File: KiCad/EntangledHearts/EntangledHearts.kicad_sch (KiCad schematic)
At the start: 42 parts, among them J1 OLED Display, J2 MPU, Q1 SFH_3711, U1 ESP32-S3-WROOM-1

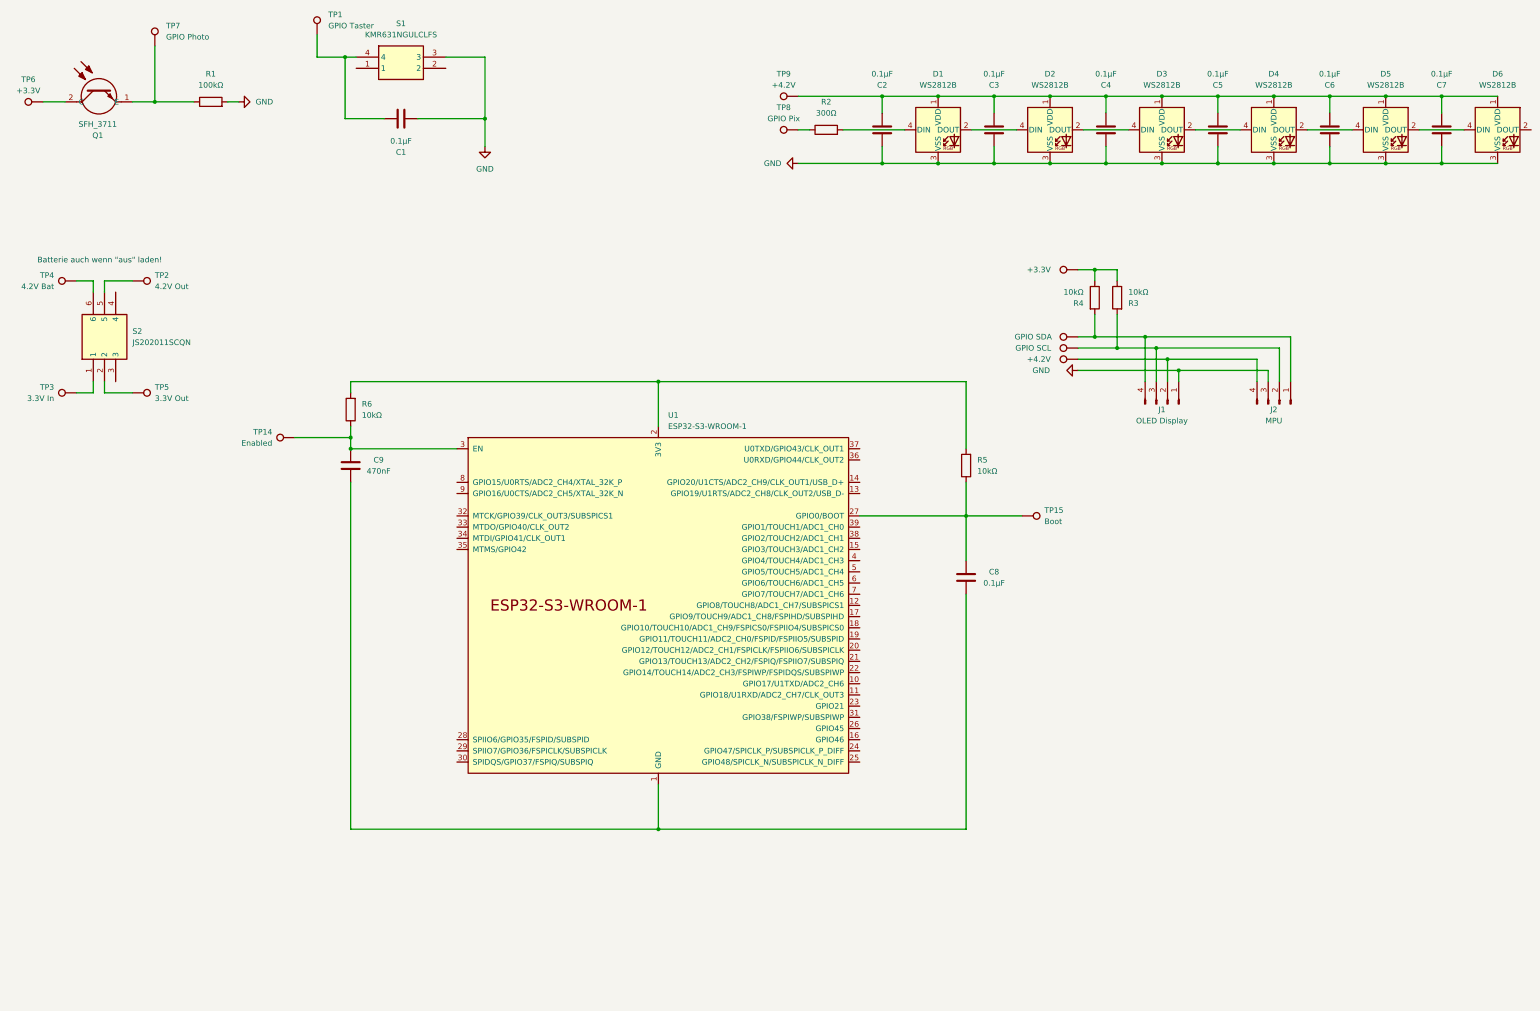
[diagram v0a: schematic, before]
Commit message: ADD: all parts added
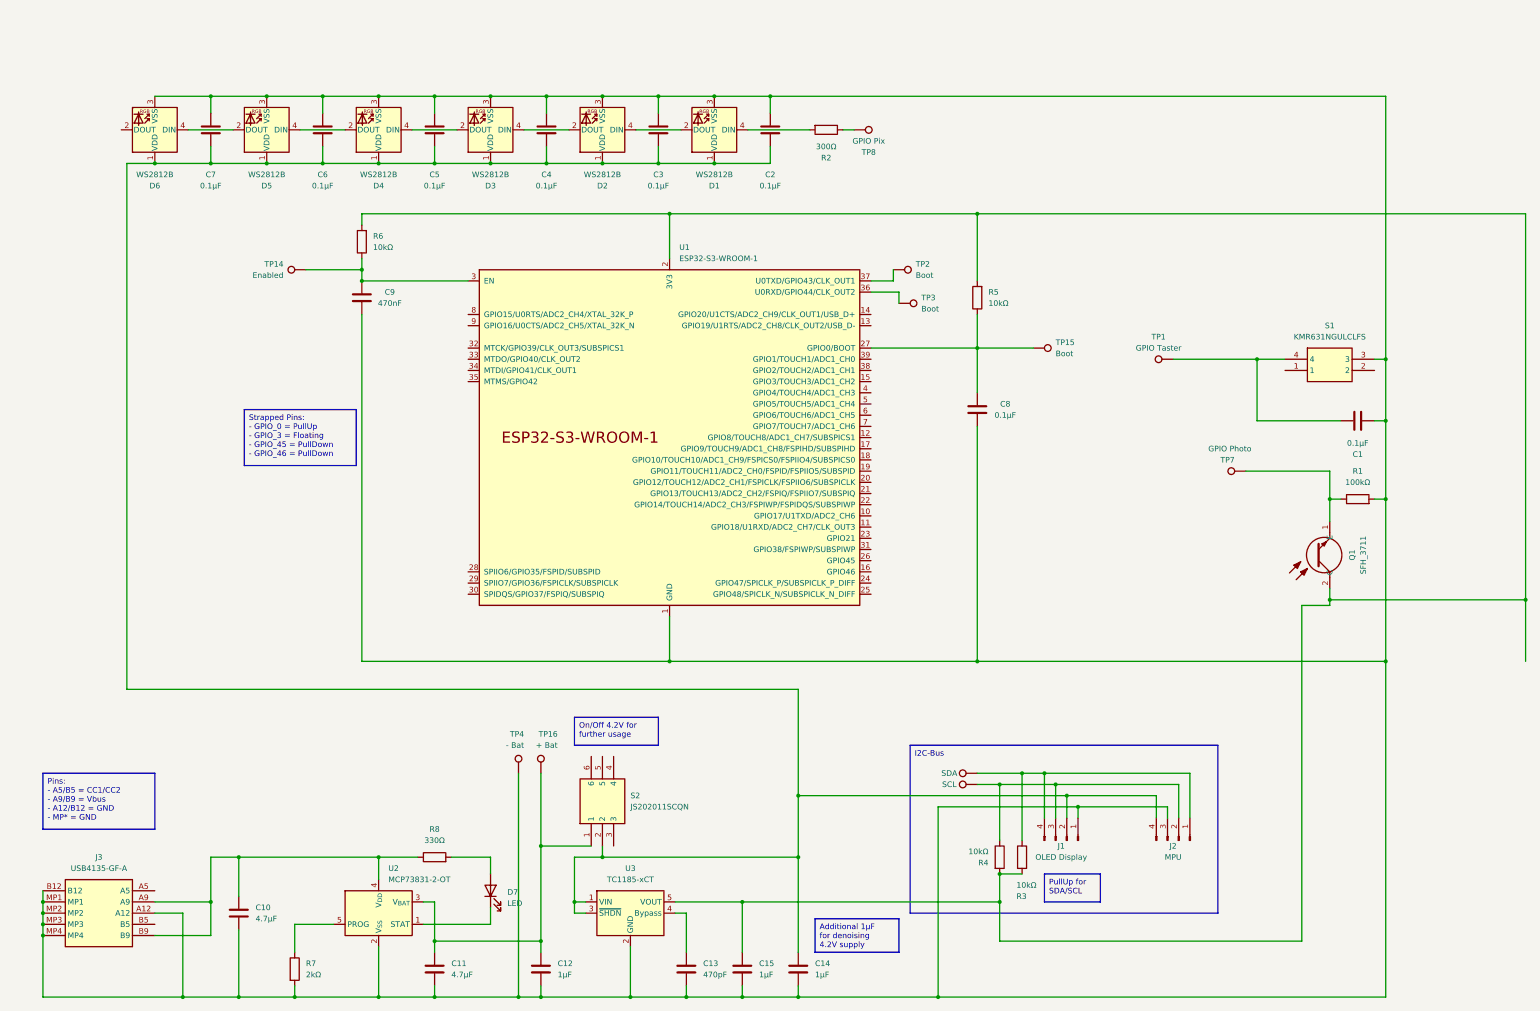
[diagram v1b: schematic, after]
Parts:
- removed TP10, TP9: +4.2V, symbol Connector:TestPoint
- removed TP13, TP6: +3.3V, symbol Connector:TestPoint
- removed TP5: 3.3V Out, symbol Connector:TestPoint
- added C10, C11: 4.7µF, symbol Device:C
- added C12, C14, C15: 1µF, symbol Device:C
- added C13: 470pF, symbol Device:C
- added D7: LED, symbol Device:LED
- added J3: USB4135-GF-A, USB4135GFA, symbol USB4135-GF-A:USB4135-GF-A
- added R7: 2kΩ, symbol Device:R
- added R8: 330Ω, symbol Device:R
- added TP16: + Bat, symbol Connector:TestPoint
- added U2: MCP73831-2-OT, Package_TO_SOT_SMD:SOT-23-5, symbol Battery_Management:MCP73831-2-OT
- added U3: TC1185-xCT, Package_TO_SOT_SMD:SOT-23-5, symbol Regulator_Linear:TC1185-xCT
- TP11: value GPIO SCL -> SCL
- TP12: value GPIO SDA -> SDA
- TP2: value 4.2V Out -> Boot
- TP3: value 3.3V In -> Boot
- TP4: value 4.2V Bat -> - Bat
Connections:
- net GND is gone; now on an unnamed net: C1.2, C2.2, C3.2, C4.2, C5.2, C6.2, C7.2, D1.3 (VSS), D2.3 (VSS), D3.3 (VSS), D4.3 (VSS), D5.3 (VSS), D6.3 (VSS), J1.1 (Pin_1), J2.3 (Pin_3), R1.2, S1.3
- net at TP2.1: now also U1.37 (U0TXD/GPIO43/CLK_OUT1); no longer S2.5
- net at J1.3 (Pin_3), J2.2 (Pin_2), TP11.1: now also R4.1; no longer R3.2
- net at J1.2 (Pin_2), J2.4 (Pin_4): now also C2.1, C3.1, C4.1, C5.1, C6.1, C7.1, D1.1 (VDD), D2.1 (VDD), D3.1 (VDD), D4.1 (VDD), D5.1 (VDD), D6.1 (VDD), S2.2, C14.1, U3.1 (VIN), U3.3 (~{SHDN})
- net at J1.4 (Pin_4), J2.1 (Pin_1), TP12.1: now also R3.1; no longer R4.2
- net at C8.1, C9.1, U1.1 (GND)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: now also TP4.1, C10.2, C11.2, C12.2, C13.2, C14.2, C15.2, J3.A12, J3.B12, J3.MP1, J3.MP2, J3.MP3, J3.MP4, R7.2, U2.2 (V_{SS}), U3.2 (GND)
- net at R5.2, R6.2, U1.2 (3V3): now also Q1.2 (C), R3.2, R4.2, C15.1, U3.5 (VOUT)
- net at U1.36 (U0RXD/GPIO44/CLK_OUT2): now also TP3.1
- net at S2.6: no longer TP4.1
- net at S2.1: now also C11.1, C12.1, TP16.1, U2.3 (V_{BAT}); no longer TP3.1
- new net: C10.1, J3.A9, J3.B9, R8.1, U2.4 (V_{DD})
- new net: C13.1, U3.4 (Bypass)
- new net: D7.1 (K), U2.1 (STAT)
- new net: D7.2 (A), R8.2
- new net: R7.1, U2.5 (PROG)
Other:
- note removed: "Batterie auch wenn "aus" laden!"
- moved on the sheet: C1, C2, C3, C4, C5, C6, C7, C8, C9, D1, D2, D3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

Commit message: ADD: final touches for first plot
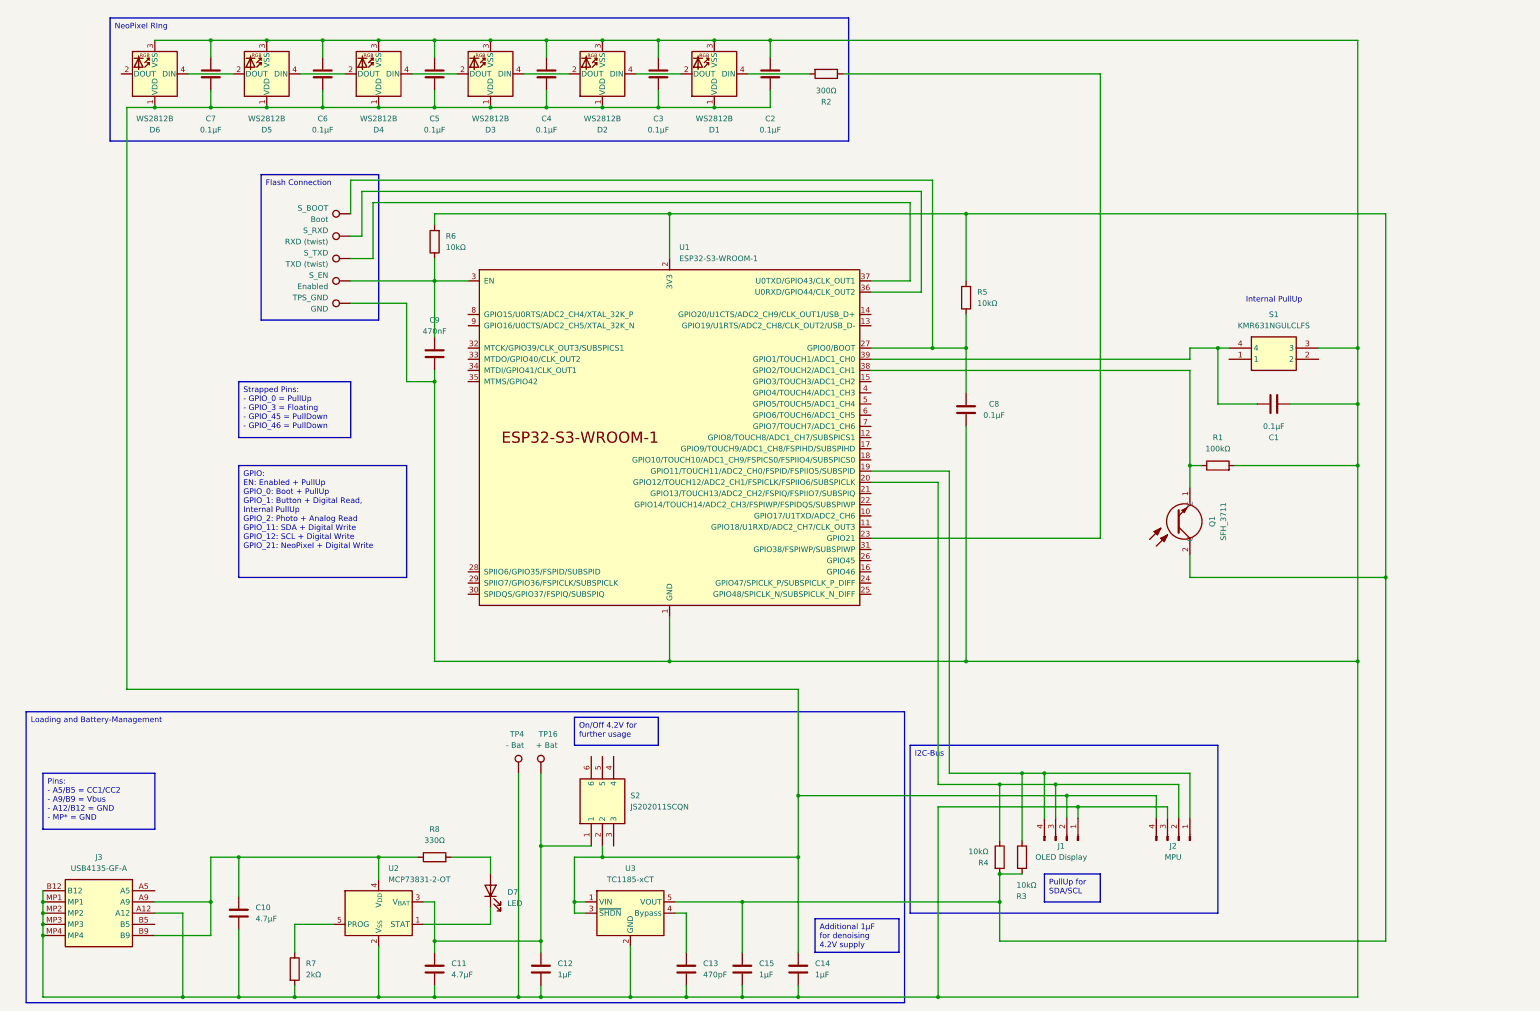
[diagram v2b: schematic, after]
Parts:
- removed TP1: GPIO Taster, symbol Connector:TestPoint
- removed TP11: SCL, symbol Connector:TestPoint
- removed TP12: SDA, symbol Connector:TestPoint
- removed TP14: Enabled, symbol Connector:TestPoint
- removed TP15, TP2, TP3: Boot, symbol Connector:TestPoint
- removed TP7: GPIO Photo, symbol Connector:TestPoint
- removed TP8: GPIO Pix, symbol Connector:TestPoint
- added S_BOOT: Boot, symbol Connector:TestPoint
- added S_EN: Enabled, symbol Connector:TestPoint
- added S_RXD: RXD (twist), symbol Connector:TestPoint
- added S_TXD: TXD (twist), symbol Connector:TestPoint
- added TPS_GND: GND, symbol Connector:TestPoint
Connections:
- net at U1.36 (U0RXD/GPIO44/CLK_OUT2): now also S_RXD.1
- net at C1.1, S1.4: now also U1.39 (GPIO1/TOUCH1/ADC1_CH0)
- net at C1.2, C10.2, C11.2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: now also TPS_GND.1
- net at Q1.1 (E), R1.1: now also U1.38 (GPIO2/TOUCH2/ADC1_CH1)
- net at J1.3 (Pin_3), J2.2 (Pin_2), R4.1: now also U1.20 (GPIO12/TOUCH12/ADC2_CH1/FSPICLK/FSPIIO6/SUBSPICLK)
- net at C9.2, R6.1, U1.3 (EN): now also S_EN.1
- net at J1.4 (Pin_4), J2.1 (Pin_1), R3.1: now also U1.19 (GPIO11/TOUCH11/ADC2_CH0/FSPID/FSPIIO5/SUBSPID)
- net at C8.2, R5.1, U1.27 (GPIO0/BOOT): now also S_BOOT.1
- net at R2.1: now also U1.23 (GPIO21)
- net at U1.37 (U0TXD/GPIO43/CLK_OUT1): now also S_TXD.1
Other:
- note added: "Internal PullUp"
- moved on the sheet: C1, C2, C3, C4, C5, C6, C7, C8, C9, D1, D2, D3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
